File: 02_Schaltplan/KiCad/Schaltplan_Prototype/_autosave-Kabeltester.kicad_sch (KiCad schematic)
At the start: 12 parts, among them J1 INPUT/MALE-DB9, J14 GND, J15 GND, J16 GND, J2 OUTPUT/FEMALE-DB9, J4 VCC

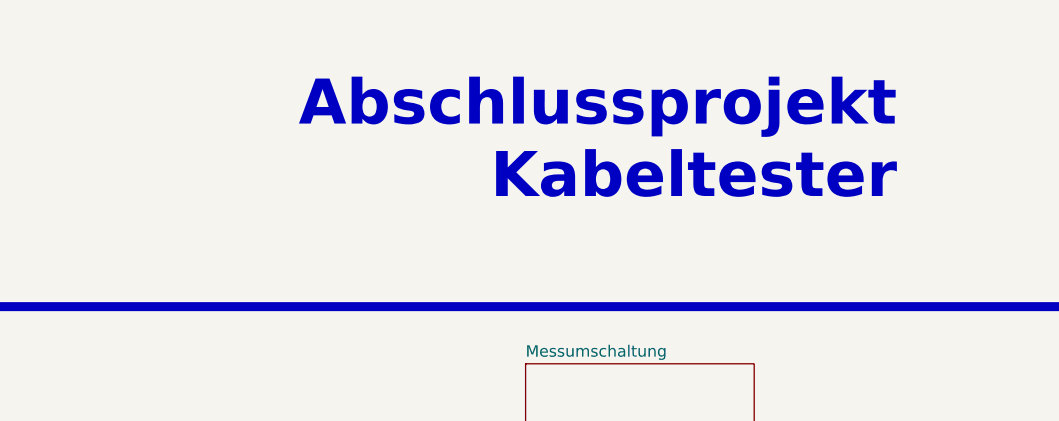
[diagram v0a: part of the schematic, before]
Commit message: ADD
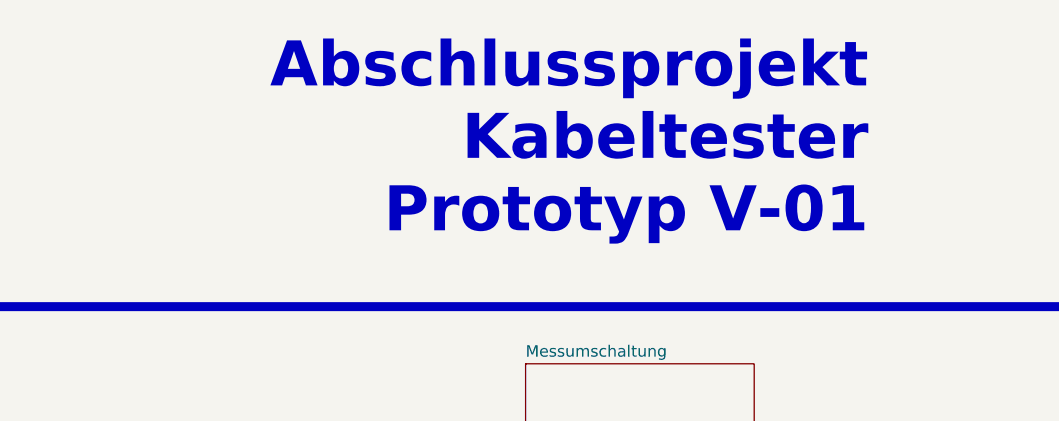
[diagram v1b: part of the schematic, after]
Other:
- note added: "Abschlussprojekt Kabeltester Prototyp V-01"
- note removed: "Abschlussprojekt Kabeltester"
